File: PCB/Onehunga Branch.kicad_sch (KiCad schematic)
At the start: 5 parts

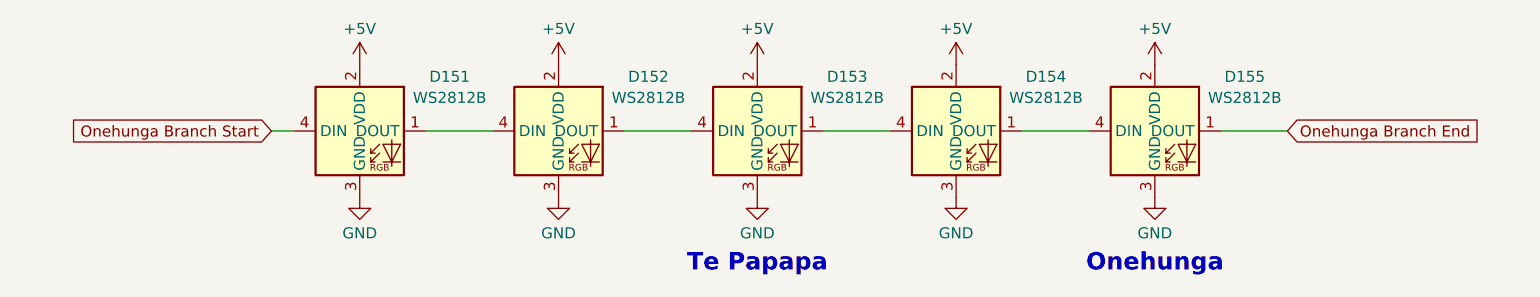
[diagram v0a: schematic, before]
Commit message: Final tweaks for V1.0.0
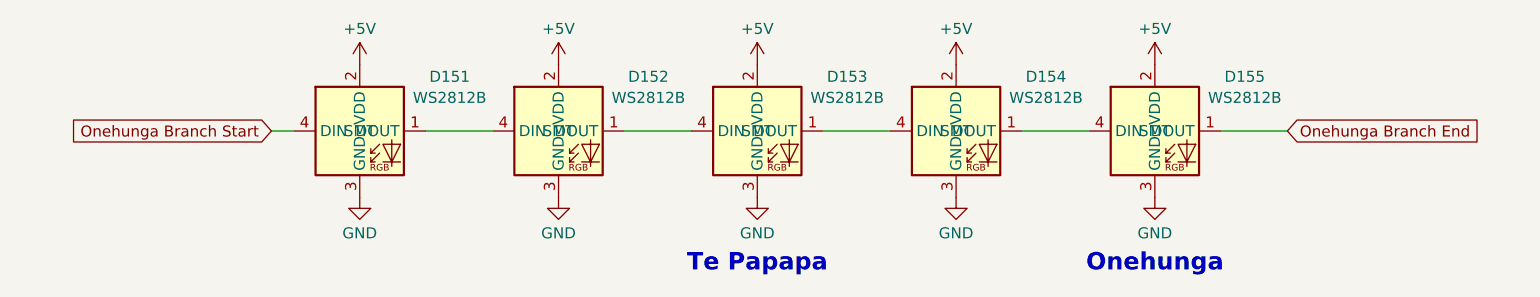
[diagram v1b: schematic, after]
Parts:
- D151, D152, D153, D154, D155: Manufacturer (none) -> XINGLIGHT; Part (none) -> XL-1615RGBC-WS2812B; Process (none) -> SMT
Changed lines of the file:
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@@
+			)
+		)
+		(property "Part" "XL-1615RGBC-WS2812B"
+			(at 93.98 25.4 0)
+			(effects
+				(font
+					(size 1.27 1.27)
+				)
+				(hide yes)
+			)
+		)
+		(property "Manufacturer" "XINGLIGHT"
+			(at 93.98 25.4 0)
+			(effects
+				(font
+					(size 1.27 1.27)
+				)
+				(hide yes)
+			)
+		)
+		(property "PartID" ""
+			(at 93.98 25.4 0)
+			(effects
+				(font
+					(size 1.27 1.27)
+				)
+			)
+		)
+		(property "Process" "SMT"
+			(at 93.98 25.4 0)
+			(effects
+				(font
+					(size 1.27 1.27)
+				)
 			)
 		)
@@
 			)
 		)
+		(property "Part" "XL-1615RGBC-WS2812B"
+			(at 48.26 25.4 0)
+			(effects
+				(font
+					(size 1.27 1.27)
+				)
+				(hide yes)
+			)
+		)
+		(property "Manufacturer" "XINGLIGHT"
+			(at 48.26 25.4 0)
+			(effects
+				(font
+					(size 1.27 1.27)
+				)
+				(hide yes)
+			)
+		)
+		(property "PartID" ""
+			(at 48.26 25.4 0)
+			(effects
+				(font
+					(size 1.27 1.27)
+				)
+			)
+		)
+		(property "Process" "SMT"
+			(at 48.26 25.4 0)
+			(effects
+				(font
+					(size 1.27 1.27)
+				)
+			)
+		)
 		(pin "2"
 		)
@@
 			)
 		)
+		(property "Part" "XL-1615RGBC-WS2812B"
+			(at 139.7 25.4 0)
+			(effects
+				(font
+					(size 1.27 1.27)
+				)
+				(hide yes)
+			)
+		)
+		(property "Manufacturer" "XINGLIGHT"
+			(at 139.7 25.4 0)
+			(effects
+				(font
+					(size 1.27 1.27)
+				)
+				(hide yes)
+			)
+		)
+		(property "PartID" ""
+			(at 139.7 25.4 0)
+			(effects
+				(font
+					(size 1.27 1.27)
+				)
+			)
+		)
+		(property "Process" "SMT"
+			(at 139.7 25.4 0)
+			(effects
+				(font
+					(size 1.27 1.27)
+				)
+			)
+		)
 		(pin "2"
 		)
@@
 			)
 		)
+		(property "Part" "XL-1615RGBC-WS2812B"
+			(at 71.12 25.4 0)
+			(effects
+				(font
+					(size 1.27 1.27)
+				)
+				(hide yes)
+			)
+		)
+		(property "Manufacturer" "XINGLIGHT"
+			(at 71.12 25.4 0)
+			(effects
+				(font
+					(size 1.27 1.27)
+				)
+				(hide yes)
+			)
+		)
+		(property "PartID" ""
+			(at 71.12 25.4 0)
+			(effects
+				(font
+					(size 1.27 1.27)
+				)
+			)
+		)
+		(property "Process" "SMT"
+			(at 71.12 25.4 0)
+			(effects
+				(font
+					(size 1.27 1.27)
+				)
+			)
+		)
 		(pin "2"
 		)
@@
 			)
 		)
+		(property "Part" "XL-1615RGBC-WS2812B"
+			(at 116.84 25.4 0)
+			(effects
+				(font
+					(size 1.27 1.27)
+				)
+				(hide yes)
+			)
+		)
+		(property "Manufacturer" "XINGLIGHT"
+			(at 116.84 25.4 0)
+			(effects
+				(font
+					(size 1.27 1.27)
+				)
+				(hide yes)
+			)
+		)
+		(property "PartID" ""
+			(at 116.84 25.4 0)
+			(effects
+				(font
+					(size 1.27 1.27)
+				)
+			)
+		)
+		(property "Process" "SMT"
+			(at 116.84 25.4 0)
+			(effects
+				(font
+					(size 1.27 1.27)
+				)
+			)
+		)
